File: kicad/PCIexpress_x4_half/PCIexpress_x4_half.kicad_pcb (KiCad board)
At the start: 4 copper layers, 167.7 x 111.2 mm, 18 parts, among them J1 PCIexpress_bracket, J2 PCIexpress_x4

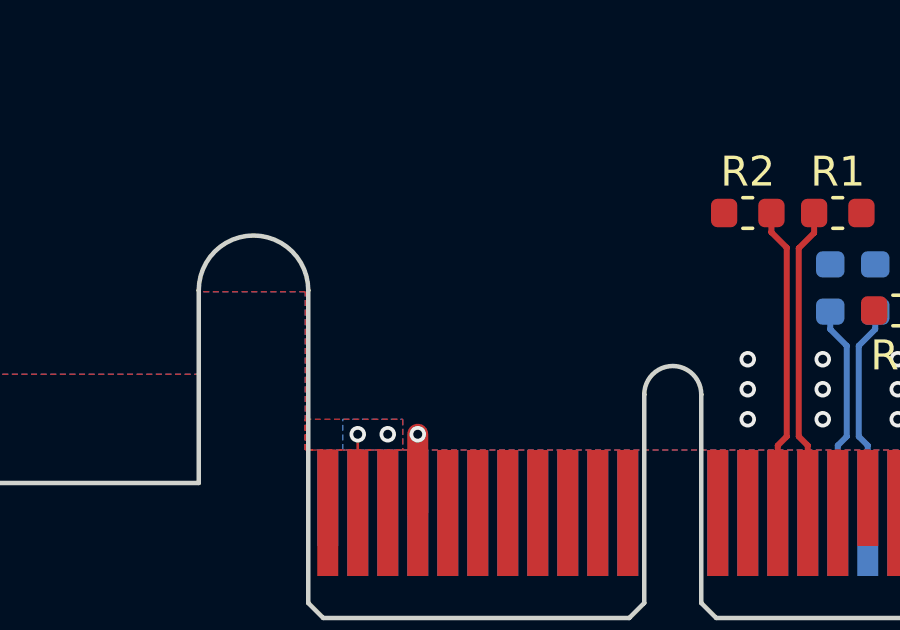
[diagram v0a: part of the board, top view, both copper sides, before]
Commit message: update
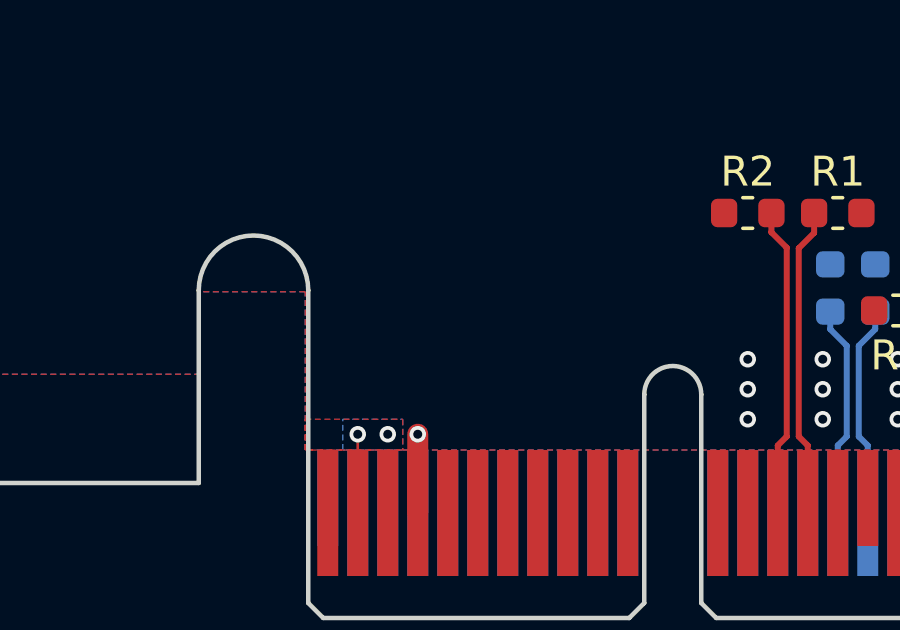
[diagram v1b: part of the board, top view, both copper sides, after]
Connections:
- net /~PERST renamed /~{PERST}
- net /~PRSNT1 renamed /~{PRSNT1}
- net /~PRSNT2x1 renamed /~{PRSNT2x1}
- net /~PRSNT2x4 renamed /~{PRSNT2x4}
- net /~TRST renamed /~{TRST}
- net /~WAKE renamed /~{WAKE}
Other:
- net class Default removed
- net class Diff-100-PCIe removed
- net class JLC2313-100d-3.5 removed
- net class JLC2313-100d-4 removed
- net class JLC7628-100d-8 removed
